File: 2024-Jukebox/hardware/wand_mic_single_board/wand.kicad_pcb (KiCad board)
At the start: 4 copper layers, 17.5 x 47 mm, 52 parts, among them J1 USB_C_Receptacle_USB2.0, J10 Conn_01x03, J4 Conn_01x02, J6 Conn_01x01, J9 Conn_01x02, Q1 MUN5214DW1T1G, Q3 CJ3139K, U1 CP2104, U2 ESP32-PICO-D4, U3 ICM-20948, U4 TP4065-4.2V, U5 TLV76718DRVx, U6 LY68L6400SLIT, U7 PCA9306, U9 TLV76733DRVx

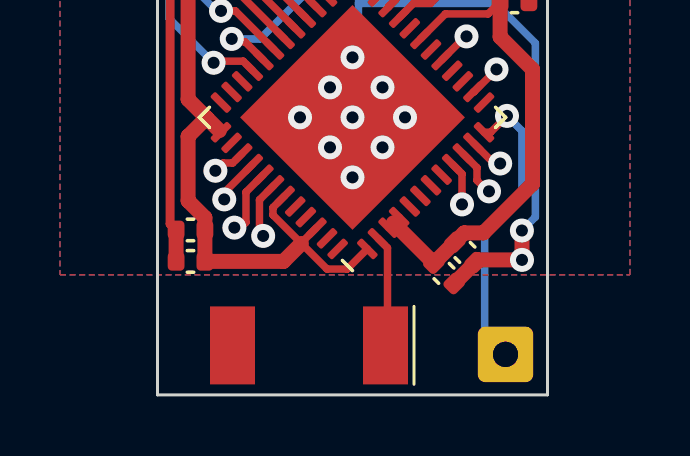
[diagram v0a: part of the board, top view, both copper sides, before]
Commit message: Updated wand PCB
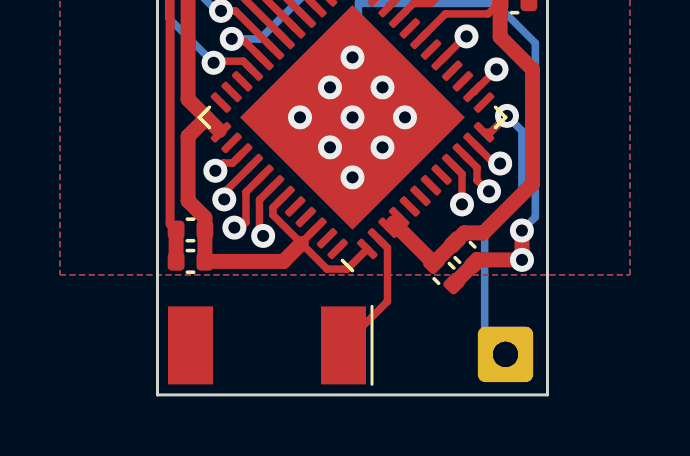
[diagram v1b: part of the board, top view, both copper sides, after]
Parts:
- moved AE1 1.40 mm to (5.90, 45.4)
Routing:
- net Net-(AE1-FEED): track 3.73 -> 4.31 mm
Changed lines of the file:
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@@
   (net 92 "Net-(J6-Pin_1)")
   (footprint "AlexCustom:NN01-102" (layer "F.Cu")
-    (at 7.3 45.35 180)
+    (at 5.9 45.35 180)
     (property "Sheetfile" "wand.kicad_sch")
     (property "Sheetname" "")
@@
         (effects (font (size 1 1) (thickness 0.15)) (justify mirror))
     )
-    (fp_text value "Conn_01x02" (at -20.25 -5.07) (layer "B.Fab")
+    (fp_text value "Conn_01x02" (at 2.37 -1.6 90) (layer "B.Fab")
         (effects (font (size 1 1) (thickness 0.15)) (justify mirror))
     )
@@
         (effects (font (size 1 1) (thickness 0.15)) (justify mirror))
     )
-    (fp_text value "Conn_01x02" (at -20.25 -5.07) (layer "B.Fab")
+    (fp_text value "Conn_01x02" (at -2.17 -1.2 90) (layer "B.Fab")
         (effects (font (size 1 1) (thickness 0.15)) (justify mirror))
     )
@@
       (net 65 "+BATT") (pinfunction "Pin_2") (pintype "passive"))
     (model "${KIPRJMOD}/cad/wand_battery_switch.step"
-      (offset (xyz -3.75 8 2))
+      (offset (xyz -3.75 8 2.5))
       (scale (xyz 1 1 1))
       (rotate (xyz 0 0 0))
@@
   (segment (start 7.397157 25.047157) (end 7.667157 24.777157) (width 0.2) (layer "F.Cu") (net 78))
   (segment (start 10.5125 19) (end 11.23 19.7175) (width 0.2) (layer "F.Cu") (net 78))
+  (segment (start 9.916542 42.098523) (end 9.916542 43.883458) (width 0.25) (layer "F.Cu") (net 79))
   (segment (start 9.598528 41.780509) (end 9.916542 42.098523) (width 0.25) (layer "F.Cu") (net 79))
-  (segment (start 9.916542 45.283458) (end 9.85 45.35) (width 0.25) (layer "F.Cu") (net 79))
-  (segment (start 9.916542 42.098523) (end 9.916542 45.283458) (width 0.25) (layer "F.Cu") (net 79))
+  (segment (start 9.916542 43.883458) (end 8.45 45.35) (width 0.25) (layer "F.Cu") (net 79))
   (segment (start 13.264986 40.214986) (end 12.899873 39.849873) (width 0.25) (layer "F.Cu") (net 80))
   (segment (start 14.28 17.73) (end 14.35 17.8) (width 0.25) (layer "F.Cu") (net 80))
